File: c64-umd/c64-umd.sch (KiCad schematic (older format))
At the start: 6 parts

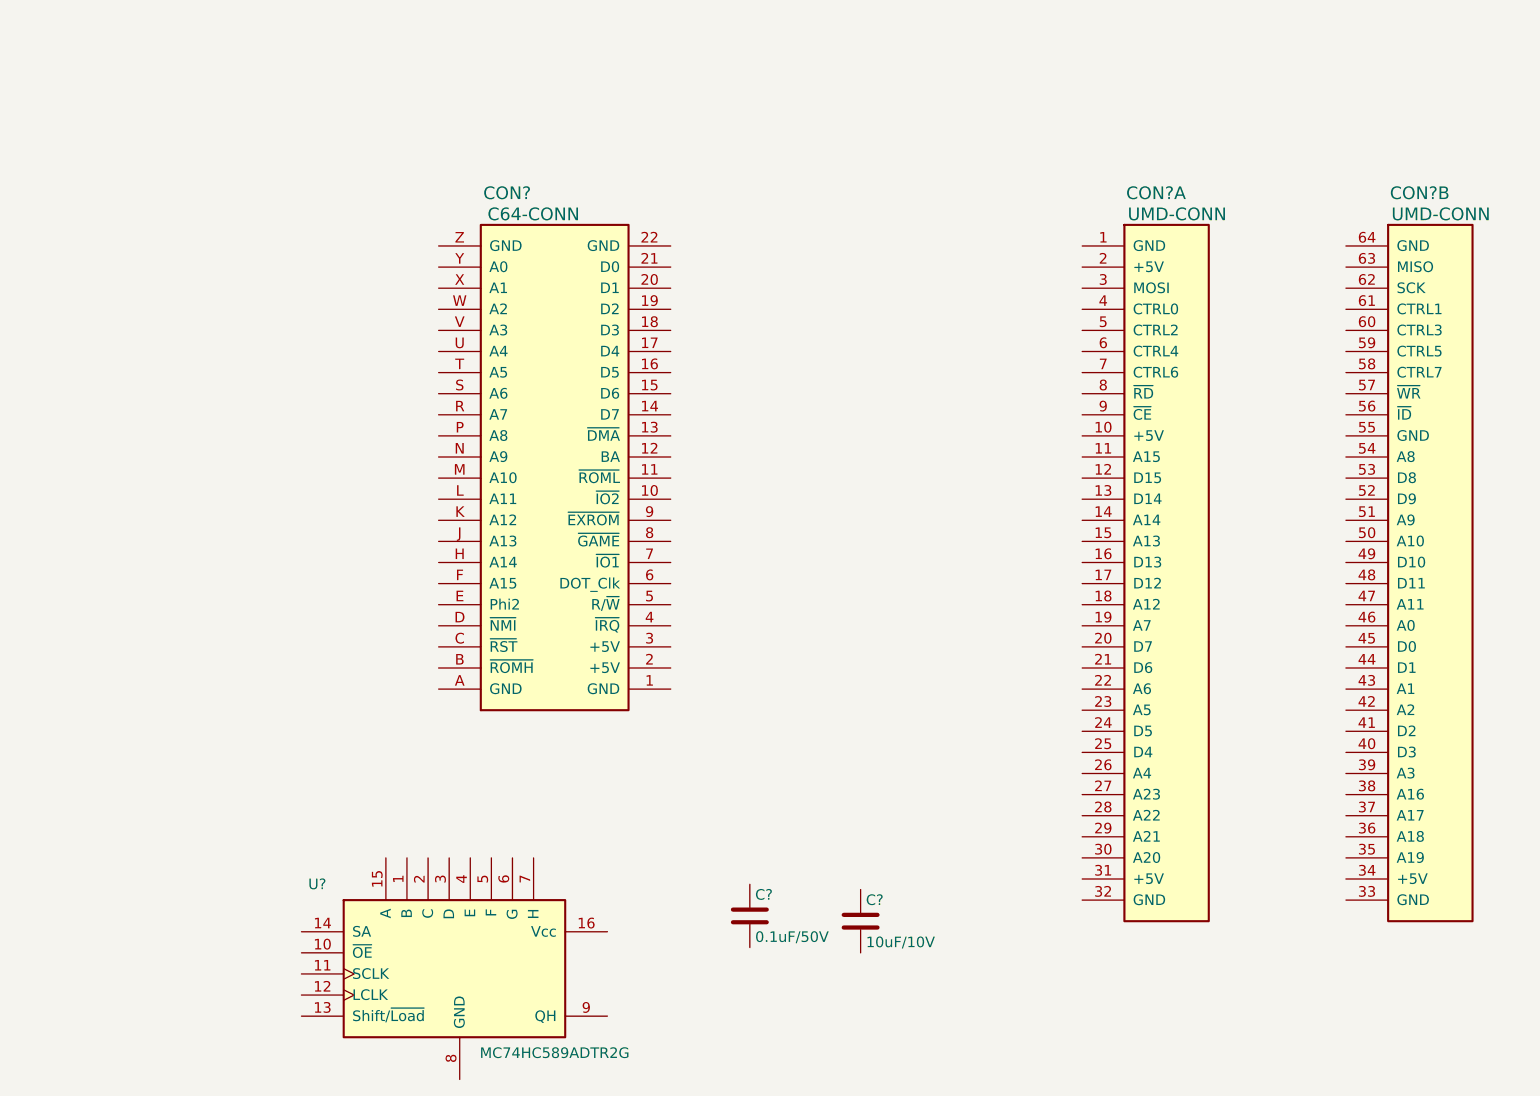
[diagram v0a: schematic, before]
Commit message: prelim sch done
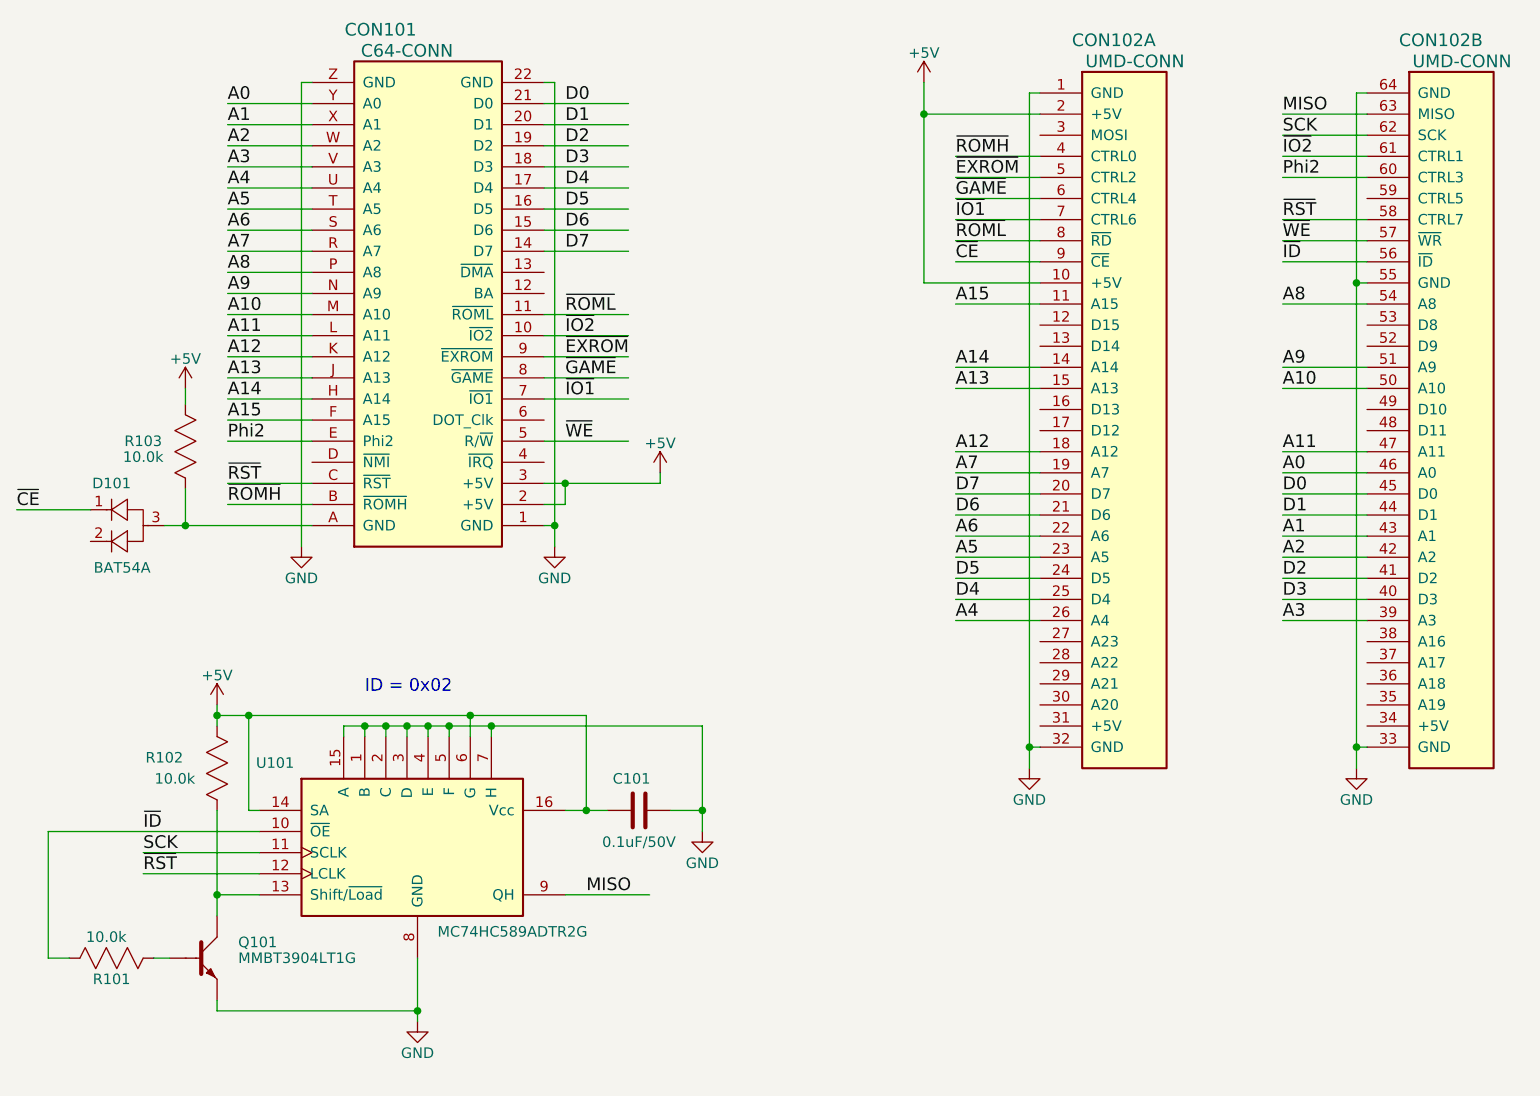
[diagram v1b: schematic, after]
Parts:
- removed C?: 10uF/10V, db-smt:0805, symbol C_0805
- added D101: BAT54A, db-smt:SOT23, symbol BAT54A
- added Q101: MMBT3904LT1G, SOT-23, symbol MMBT3904LT1G
- added R101, R102, R103: 10.0k, db-smt:0603, symbol R_0603
- gave numbers to parts that had none: 4
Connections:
- net labels added: +5V, A0, A1, A10, A11, A12, A13, A14, A15, A2, A3, A4, A5, A6, A7, A8, A9, D0, D1, D2, D3, D4, D5, D6, D7, GND, MISO, Phi2, SCK, ~CE, ~EXROM, ~GAME, ~ID, ~IO1, ~IO2, ~ROMH, ~ROML, ~RST, ~WE
- wire segments 0 -> 143
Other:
- note added: "ID = 0x02"
- moved on the sheet: C101, CON101, CON102A, CON102B, U101
